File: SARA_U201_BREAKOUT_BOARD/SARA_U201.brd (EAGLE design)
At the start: 103.9 x 69.8 mm, 57 parts, among them IC1 TS3USB221ERSER, J6 -, T1 BC847, U1 LT1764AEQ#PBF, U2 SN74AVC4T774PW, U3 SN74AVC4T774PW, U4 SARA-U201-03B, X1 CCM03-3013LFT_R102

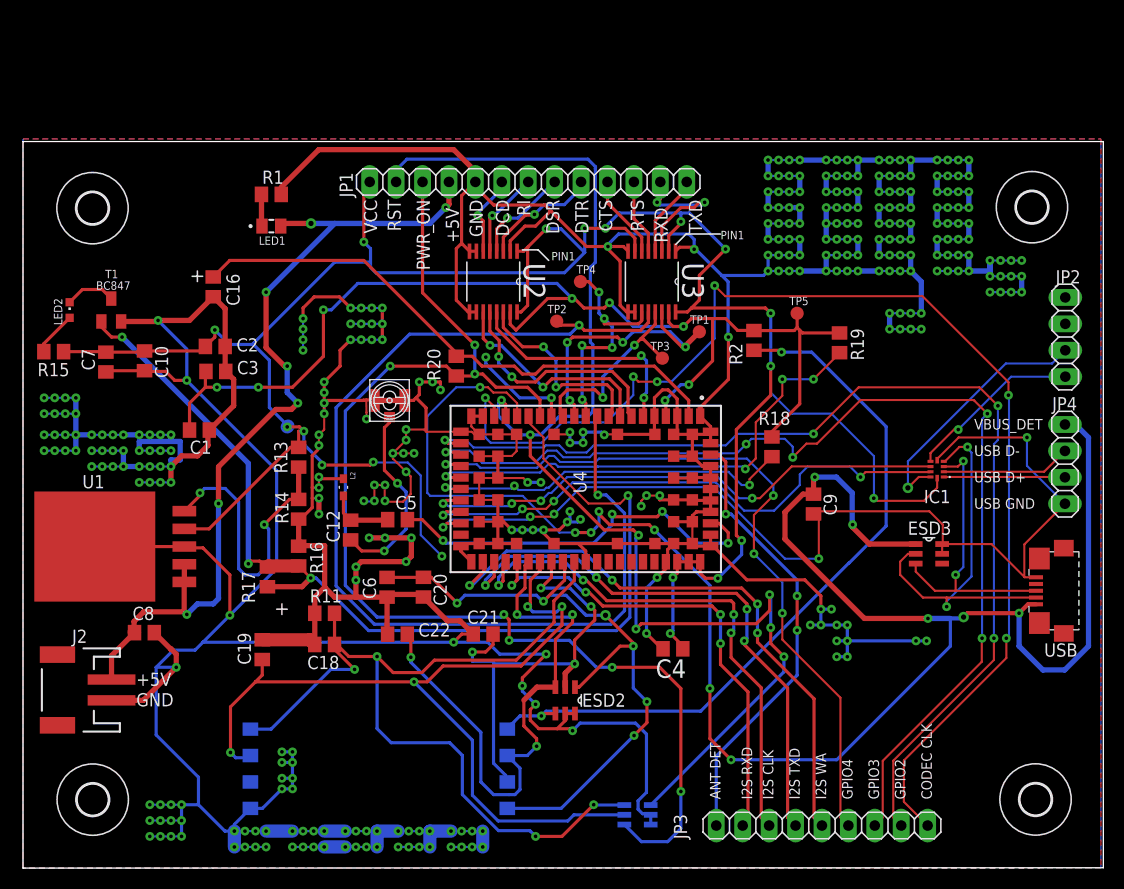
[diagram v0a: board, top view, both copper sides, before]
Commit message: Added Teensy, MIC, Boost connectors along with some layout changes with USB switch and rerouting all the connections
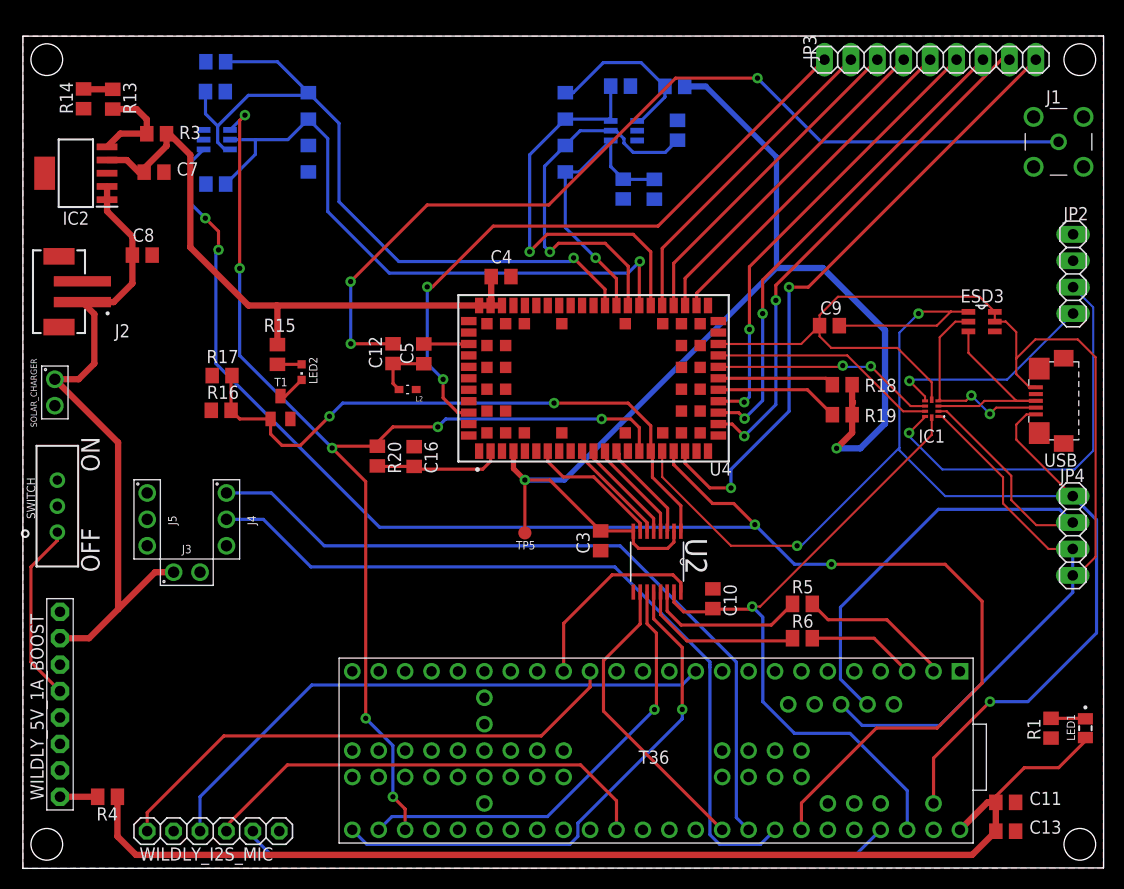
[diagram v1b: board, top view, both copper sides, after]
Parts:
- removed C1, C2: 100nF, rcl:C0805
- removed H1, H2, H3, H4: MOUNT-HOLE3.0, holes:3,0
- removed J6: -, Arduino-connectors:U.FL-R-SMT-1(60)
- removed JP1: (no value), pinhead:1X13
- removed TP1, TP2, TP3, TP4: TPB1,27, testpad:B1,27
- removed U1: LT1764AEQ#PBF, LT1764AEQ_PBF:DDPAK-5_Q
- removed U3: SN74AVC4T774PW, SN74AVC4T774PW:SOP65P640X120-16N
- added C11, C13: (no value), rcl:C0805
- added IC2: MCP1826T-3302E_DC, MCP1826T-3302E_DC:SOT127P706X180-6N
- added J1: SMA_CONNECTOR, SMA_CONNECTOR:LPRS_SMA_CONNECTOR
- added J3, SOLAR_CHARGER: 61300211121, 61300211121:61300211121
- added J4, J5: 61300311121, 61300311121:61300311121
- added R3: 100K, rcl:R0805
- added R4, R5, R6: 0R, adafruit:M0805
- added SWITCH: GSM Power, EG1218:3PIN_SLIDE_SWITCH
- added U$1: TEENSY3_6--ALLPINS, Teensy_3_6:T36
- added WILDLY_5V_1A_BOOST: (no value), adafruit:1X08-BIG
- added WILDLY_I2S_MIC: (no value), adafruit:1X06
- C7: value 10uF -> 2.2uF
- J2: value (none) -> B2B-PH-SM4-TB(LF)(SN); device SparkFun-Connectors:JST-2-SMD -> B2B-PH-SM4-TB_LF__SN_:JST_B2B-PH-SM4-TB(LF)(SN)
- R13: value 6K8 -> 10K
- R14: value 3K9 -> 1K
- U2: value SN74AVC4T774PW -> TXB0106PWR; device SN74AVC4T774PW:SOP65P640X120-16N -> TXB0106PWR:SOP65P640X120-16N
- moved LED1 92.0 mm to (102.1, 13.4), turned to 270 degrees
- moved R1 90.8 mm to (98.8, 13.4), turned to 90 degrees
- moved ESD1 76.5 mm to (18.6, 70.0), turned to 0 degrees
- moved JP3 74.4 mm to (87.2, 77.7)
- moved X1 61.4 mm to (39.8, 70.7)
- moved C10 59.2 mm to (66.3, 25.9), turned to 90 degrees
- moved C22 56.9 mm to (57.4, 75.2), flipped to the bottom
- moved ESD2 55.1 mm to (57.8, 70.9), flipped to the bottom, turned to 180 degrees
- moved C18 54.2 mm to (18.5, 74.7), flipped to the bottom
- moved R11 54.0 mm to (18.5, 77.5), flipped to the bottom, turned to 180 degrees
- moved C21 51.9 mm to (62.9, 70.9), flipped to the bottom, turned to 270 degrees
- moved C6 46.1 mm to (60.7, 65.3), flipped to the bottom
- moved C19 45.0 mm to (18.5, 65.8), flipped to the bottom, turned to 180 degrees
- moved R14 44.5 mm to (5.82, 74.0)
- moved C20 42.8 mm to (57.7, 65.3), flipped to the bottom
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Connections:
- removed net DCD: JP1.8, U2.6
- removed net DSR: JP1.6, U2.4
- removed net DTR: JP1.5, U2.3
- new net 5V_EN: SWITCH.1, WILDLY_5V_1A_BOOST.5
- new net 5V_SUPPLY: R4.2, WILDLY_5V_1A_BOOST.1
- new net FUEL_GAUGE_SCL: J4.2, U$1.19
- new net FUEL_GAUGE_SDA: J4.1, U$1.18
- new net LB: WILDLY_5V_1A_BOOST.3
- new net MIC_BCLK: U$1.9, WILDLY_I2S_MIC.3
- new net MIC_DOUT: U$1.13, WILDLY_I2S_MIC.4
- new net MIC_LRCLK: U$1.23, WILDLY_I2S_MIC.5
- new net N$2: IC2.5, R13.2, R3.1
- new net N$4: WILDLY_5V_1A_BOOST.6
- new net STAT: U$1.24, U2.16
- new net V+: C8.1, IC2.1, IC2.2, J2.1, J3.1, SOLAR_CHARGER.1, WILDLY_5V_1A_BOOST.7
- new net VDD: C4.2, C7.1, IC2.4, R15.2, R3.2, U4.51, U4.52, U4.53
- net +5V: now also C11.1, C13.1, R4.1, U$1.VIN; no longer C8.1, J2.2, JP1.10, U1.1, U1.2
- net CTS: now also U$1.33, U2.12; no longer JP1.4, U3.6
- net CTS1: now also U2.5; no longer TP4.TP, U3.11
- net DCD1: no longer U2.11
- net DSR1: no longer U2.13
- net DTR1: no longer U2.14
- net GND: now also C11.2, C13.2, IC2.3, IC2.6, J1.2, J1.3, J1.4, J1.5, J2.2, J3.2, SOLAR_CHARGER.2, SWITCH.2, U$1.G0, U$1.G1, U$1.G2, U$1.G3, U$1.G4, U$1.G5, U$1.G6, WILDLY_5V_1A_BOOST.2, WILDLY_5V_1A_BOOST.4, WILDLY_I2S_MIC.2; no longer C1.2, C2.2, J2.1, J6.GND1, J6.GND2, JP1.9, U1.3, U1.6, U2.10, U2.2, U2.7, U2.8, U3.1, U3.10, U3.8, U3.9
- net MC_USB_D+: now also U$1.D+
- net MC_USB_D-: now also U$1.D-
- net N$3: no longer U1.5
- net N$6: now also J1.1; no longer J6.SIG
- net NET_STAT: now also U2.1
- net PWR_ON: now also U$1.35; no longer JP1.11
- net RI: now also U$1.17, U2.10; no longer JP1.7, U2.5
- net RI1: now also U2.7; no longer U2.12
- net RST: now also U$1.20; no longer JP1.12
- net RTS: now also U$1.34, U2.11; no longer JP1.3, U3.5
- net RTS1: now also U2.6; no longer TP2.TP, U3.12
- net RXD: now also R6.1, R6.2, U$1.1, U2.13; no longer JP1.2, U3.3
- net RXD1: now also U2.3; no longer TP3.TP, U3.13
- net TXD: now also R5.1, R5.2, U$1.0, U2.14; no longer JP1.1, U3.4
- net TXD1: now also U2.4; no longer TP1.TP, U3.14
- net VCC: now also U$1.3V3(1), U$1.3V3(2), U$1.3V3(3), U$1.3V3(4), U2.15, WILDLY_I2S_MIC.1; no longer C2.1, C4.2, C7.1, JP1.13, R13.2, R15.2, U1.4, U2.1, U2.16, U3.16, U3.2, U3.7, U4.51, U4.52, U4.53
- net VCCINT: now also U2.2, U2.8; no longer C1.1, U2.15, U3.15
- net VUSB_DET: now also U$1.VUSB
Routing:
- net GND: track 933.3 -> 0.00 mm, vias 342 -> 0
- net VCC: track 242.6 -> 116.6 mm, vias 19 -> 1
- net RTS1: track 104.5 -> 10.3 mm, vias 2 -> 0
- net FUEL_GAUGE_SCL: track 0.00 -> 76.0 mm
- net FUEL_GAUGE_SDA: track 0.00 -> 72.4 mm
- net N$6: track 18.5 -> 88.7 mm, vias 2 -> 3
- net V+: track 0.00 -> 64.9 mm
- net MIC_LRCLK: track 0.00 -> 62.7 mm
- net VDD: track 0.00 -> 59.5 mm
- net CODEC_CLK: track 118.7 -> 61.0 mm, vias 6 -> 2
- net GPIO3: track 103.9 -> 47.0 mm, vias 5 -> 2
- net MIC_BCLK: track 0.00 -> 56.0 mm
- net N$5: track 71.3 -> 17.2 mm, vias 2 -> 0
- net GPIO2: track 103.7 -> 50.2 mm, vias 4 -> 2
- net VUSB_DET: track 182.9 -> 131.0 mm, vias 12 -> 3
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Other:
- board size 103.9 x 69.8 mm -> 103.9 x 80 mm
- board text added: "C7"
- board text added: "OFF"
- board text added: "ON"
- board text added: "R15"
- board text removed: "+5V"
- board text removed: "ANT DET"
- board text removed: "CODEC CLK"
- board text removed: "CTS"
- board text removed: "DCD"
- board text removed: "DSR"
- board text removed: "DTR"
- board text removed: "GND"
- board text removed: "GPIO2"
- board text removed: "GPIO3"
- board text removed: "GPIO4"
- board text removed: "I2S CLK"
- board text removed: "I2S RXD"
- board text removed: "I2S TXD"
- board text removed: "I2S WA"
- board text removed: "JP1"
- board text removed: "JP3"
- board text removed: "PIN1"
- board text removed: "PWR_ON"
- board text removed: "RI"
- board text removed: "RST"
- board text removed: "RTS"
- board text removed: "RXD"
- board text removed: "TXD"
- board text removed: "USB D+"
- board text removed: "USB D-"
- board text removed: "USB GND"
- board text removed: "VBUS_DET"
- board text removed: "VCC"
- board text removed: "WILDLY HSPA/GSM MODULE"
